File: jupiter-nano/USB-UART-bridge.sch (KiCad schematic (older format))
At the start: 1 part

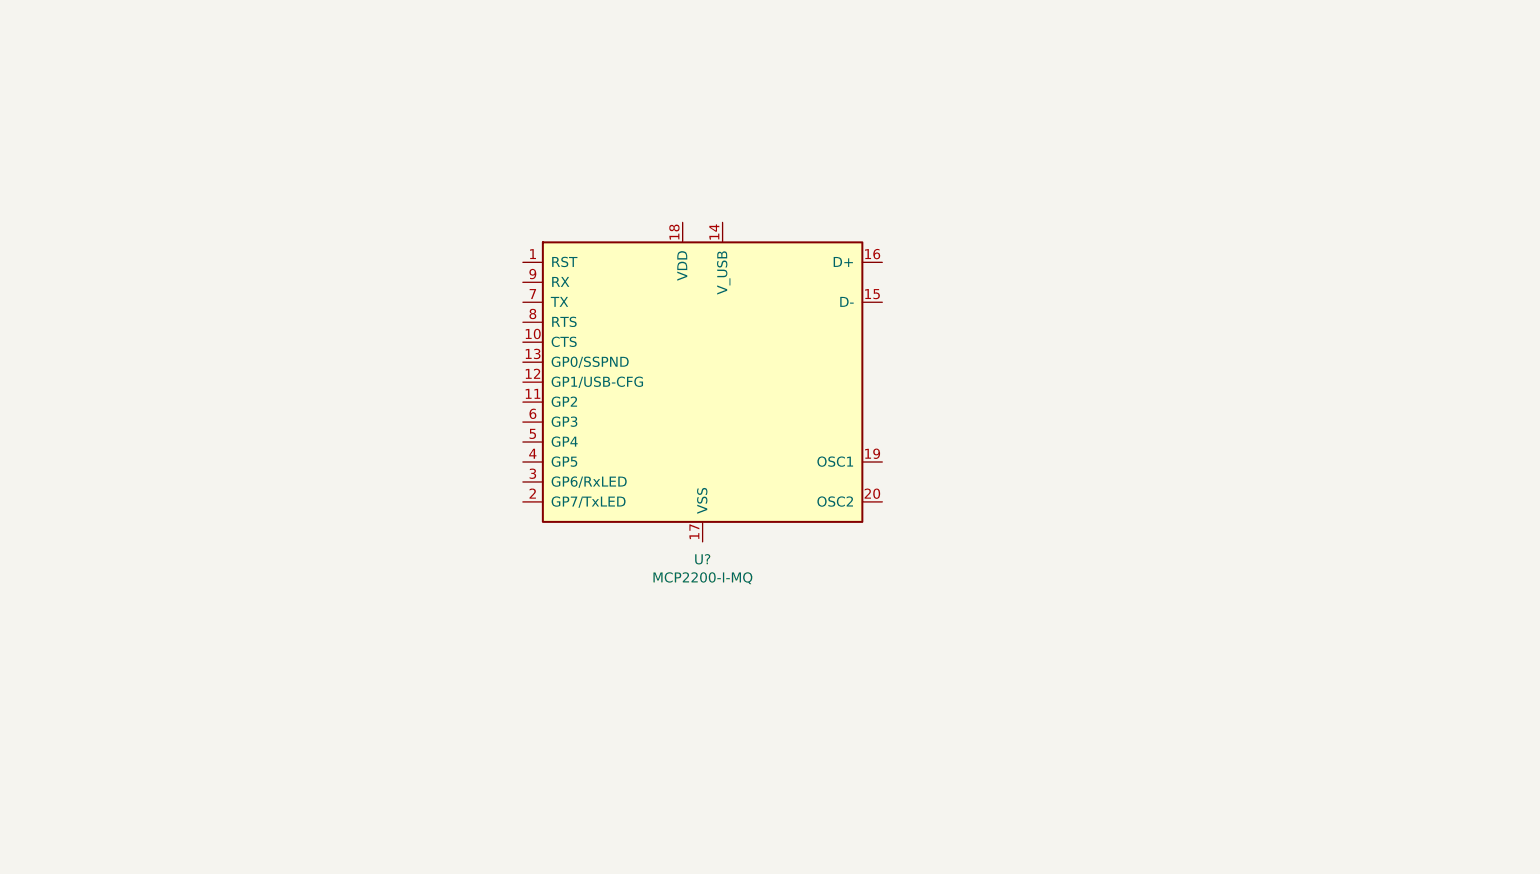
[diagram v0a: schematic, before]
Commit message: WIP, USB-UART and JTAG done
- minor clean up and SD Card form factor still left
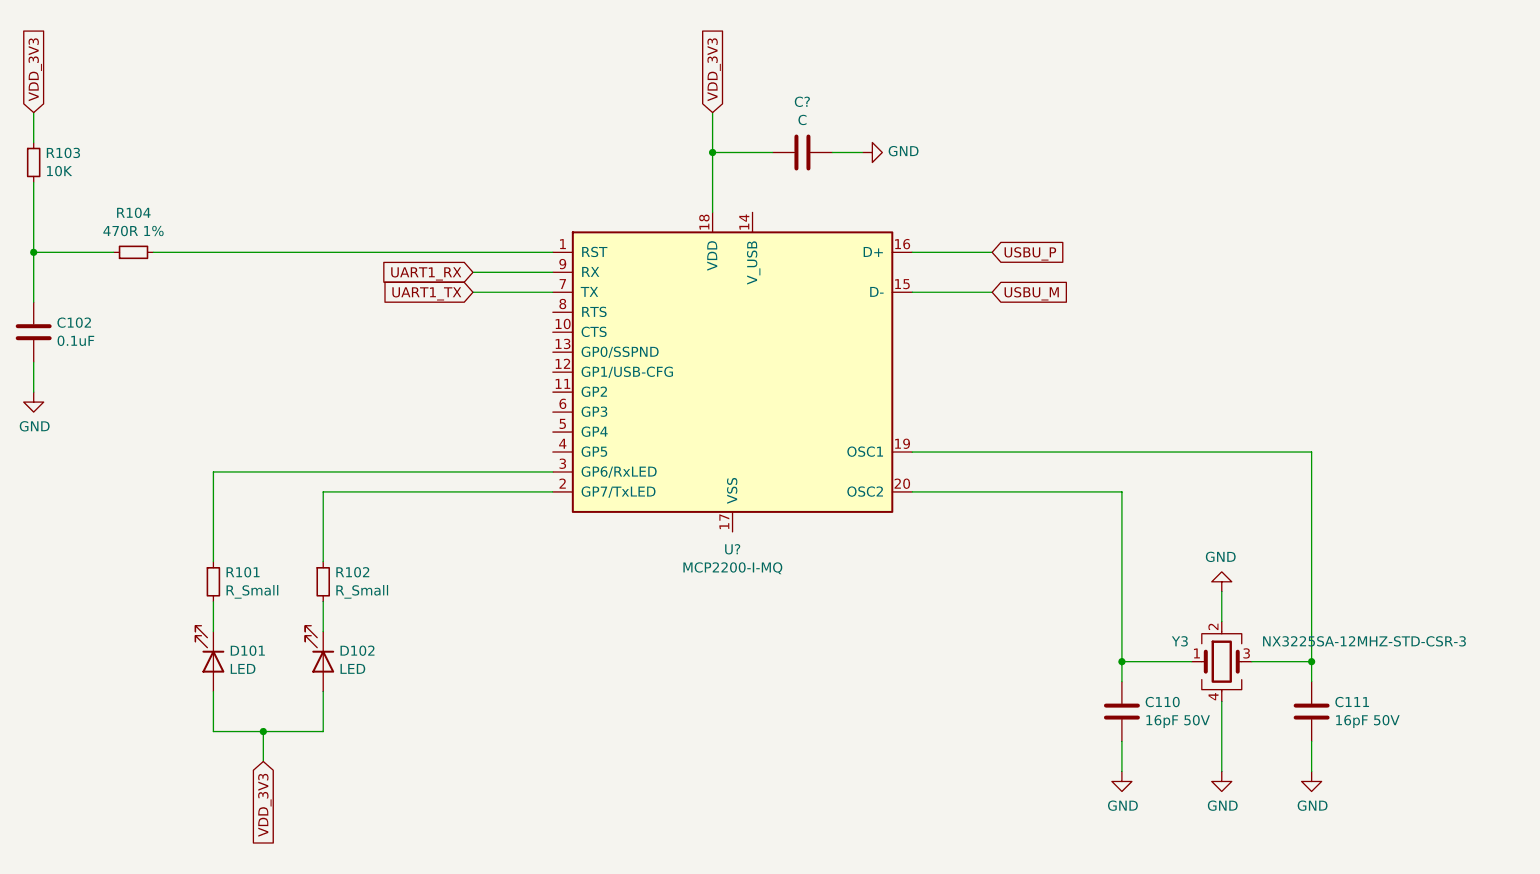
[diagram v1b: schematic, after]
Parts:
- added C102: 0.1uF, symbol Device:C
- added C110, C111: 16pF 50V, symbol Device:C
- added C?: C, symbol Device:C
- added D101, D102: LED, symbol Device:LED
- added R101, R102: R_Small, symbol Device:R_Small
- added R103: 10K, symbol Device:R_Small
- added R104: 470R 1%, symbol Device:R_Small
- added Y3: NX3225SA-12MHZ-STD-CSR-3, symbol Device:Crystal_GND24
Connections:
- net at U?.1 (RST): now also R104.2
- net USBU_M: now reaches U?.15 (D-)
- net USBU_P: now reaches U?.16 (D+)
- net VDD_3V3: now reaches U?.18 (VDD)
- net VDD_3V3: now also C?.2, D101.2 (A), D102.2 (A), R103.1
- net at U?.19 (OSC1): now also C111.1, Y3.3
- net at U?.2 (GP7/TxLED): now also R102.1
- net at U?.20 (OSC2): now also C110.1, Y3.1
- net at U?.3 (GP6/RxLED): now also R101.1
- net UART1_TX: now reaches U?.7 (TX)
- net UART1_RX: now reaches U?.9 (RX)
- new net: C102.1, R103.2, R104.1
- new net: D101.1 (K), R101.2
- new net: D102.1 (K), R102.2
- new net GND: C102.2, C110.2, C111.2, C?.1, Y3.2, Y3.4
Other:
- moved on the sheet: U?
